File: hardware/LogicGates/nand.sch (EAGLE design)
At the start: 14 parts

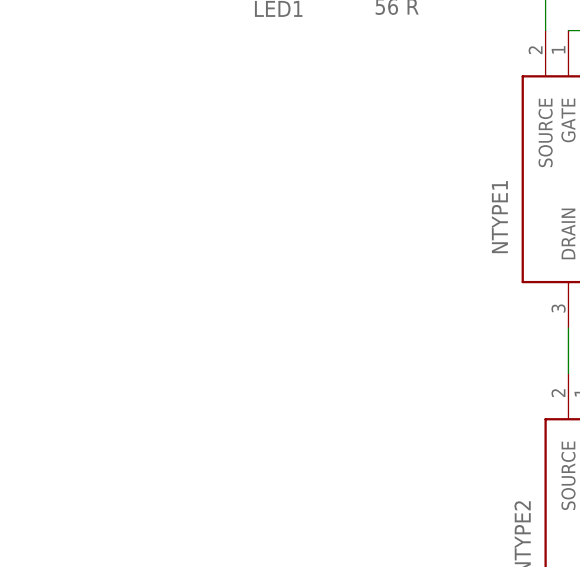
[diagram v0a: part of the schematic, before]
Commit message: made truth table a device
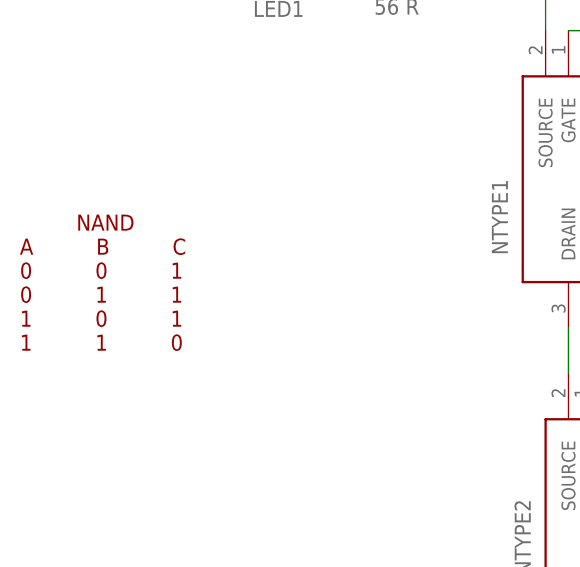
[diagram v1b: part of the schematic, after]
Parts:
- added U$2: NAND_TRUTH_TABLE, logic-gates:NAND_TRUTH_TABLE
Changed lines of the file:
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@@
 <part name="J1" library="connector" deviceset="M02" device="1X02_NO_SILK"/>
 <part name="U$1" library="logos" deviceset="CMD_C0DE_LOGO" device="CMD_CODE_LOGO_TOP_COPPER"/>
+<part name="U$2" library="logic-gates" deviceset="NAND_TRUTH_TABLE" device=""/>
 </parts>
 <sheets>
@@
 </instance>
 <instance part="U$1" gate="G$1" x="88.9" y="55.88" smashed="yes"/>
+<instance part="U$2" gate="G$1" x="-17.78" y="40.64" smashed="yes"/>
 </instances>
 <busses>
@@
 </schematic>
 </drawing>
+<compatibility>
+<note version="6.3" minversion="6.2.2" severity="warning">
+Since Version 6.2.2 text objects can contain more than one line,
+which will not be processed correctly with this version.
+</note>
+</compatibility>
 </eagle>

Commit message: make it bigger
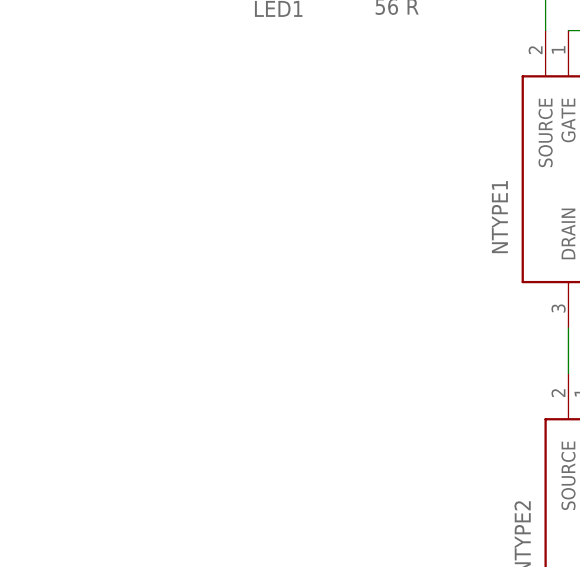
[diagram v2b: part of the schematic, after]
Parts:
- removed U$2: NAND_TRUTH_TABLE, logic-gates:NAND_TRUTH_TABLE
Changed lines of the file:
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@@
 <part name="J1" library="connector" deviceset="M02" device="1X02_NO_SILK"/>
 <part name="U$1" library="logos" deviceset="CMD_C0DE_LOGO" device="CMD_CODE_LOGO_TOP_COPPER"/>
-<part name="U$2" library="logic-gates" deviceset="NAND_TRUTH_TABLE" device=""/>
 </parts>
 <sheets>
@@
 </instance>
 <instance part="U$1" gate="G$1" x="88.9" y="55.88" smashed="yes"/>
-<instance part="U$2" gate="G$1" x="-17.78" y="40.64" smashed="yes"/>
 </instances>
 <busses>
@@
 </schematic>
 </drawing>
-<compatibility>
-<note version="6.3" minversion="6.2.2" severity="warning">
-Since Version 6.2.2 text objects can contain more than one line,
-which will not be processed correctly with this version.
-</note>
-</compatibility>
 </eagle>
